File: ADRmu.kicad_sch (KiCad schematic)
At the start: 6 parts, among them J1 DIN41612_02x16_AC_EvenPins, J2 10Vf, J3 10Vs, J4 ADR, J6 return, J7 guard

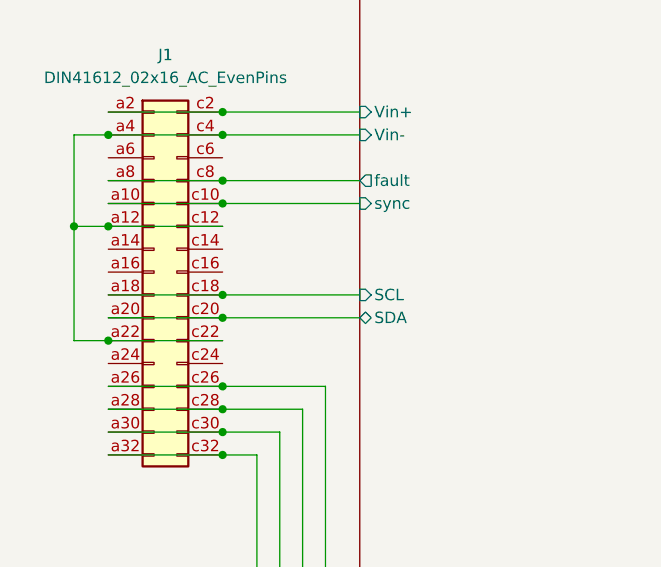
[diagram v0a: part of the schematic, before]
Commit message: asas
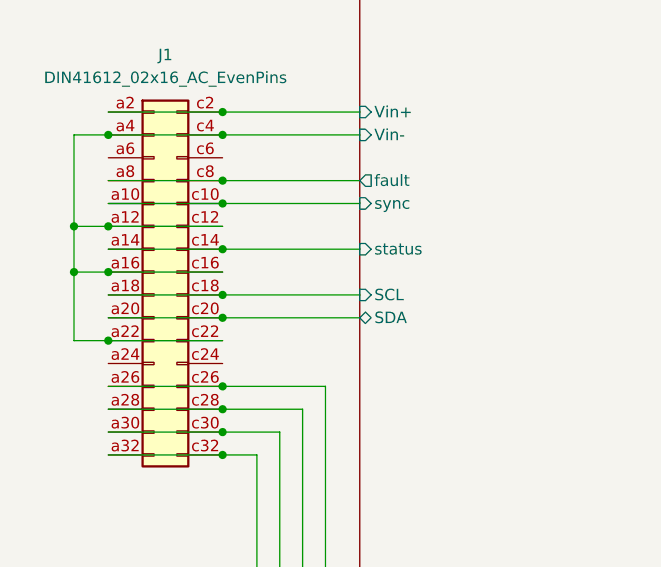
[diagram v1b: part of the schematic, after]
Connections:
- net DC-DC/Vin-: now also J1.a16 (Pin_a16), J1.c16 (Pin_c16)
- net DC-DC/status: now reaches J1.a14 (Pin_a14)
- net DC-DC/status: now also J1.c14 (Pin_c14)
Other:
- sheet DC-DC ports: added status; removed none
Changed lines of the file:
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@@
   (junction (at 68.58 82.55) (diameter 0) (color 0 0 0 0)
   )
+  (junction (at 55.88 92.71) (diameter 0) (color 0 0 0 0)
+  )
   (junction (at 55.88 100.33) (diameter 0) (color 0 0 0 0)
   )
@@
   (junction (at 68.58 105.41) (diameter 0) (color 0 0 0 0)
   )
+  (junction (at 68.58 90.17) (diameter 0) (color 0 0 0 0)
+  )
   (junction (at 68.58 85.09) (diameter 0) (color 0 0 0 0)
   )
   (junction (at 68.58 113.03) (diameter 0) (color 0 0 0 0)
   )
+  (junction (at 52.07 92.71) (diameter 0) (color 0 0 0 0)
+  )
   (junction (at 68.58 110.49) (diameter 0) (color 0 0 0 0)
   )
@@
     (stroke (width 0) (type default) (color 0 0 0 0))
   )
+  (wire (pts (xy 55.88 92.71) (xy 68.58 92.71))
+    (stroke (width 0) (type default) (color 0 0 0 0))
+  )
   (wire (pts (xy 228.6 120.65) (xy 228.6 116.84))
     (stroke (width 0) (type default) (color 0 0 0 0))
@@
     (stroke (width 0) (type default) (color 0 0 0 0))
   )
+  (wire (pts (xy 55.88 90.17) (xy 68.58 90.17))
+    (stroke (width 0) (type default) (color 0 0 0 0))
+  )
   (wire (pts (xy 55.88 77.47) (xy 52.07 77.47))
     (stroke (width 0) (type default) (color 0 0 0 0))
   )
+  (wire (pts (xy 68.58 90.17) (xy 83.82 90.17))
+    (stroke (width 0) (type default) (color 0 0 0 0))
+  )
   (wire (pts (xy 68.58 74.93) (xy 83.82 74.93))
     (stroke (width 0) (type default) (color 0 0 0 0))
@@
     (stroke (width 0) (type default) (color 0 0 0 0))
   )
+  (wire (pts (xy 52.07 92.71) (xy 52.07 100.33))
+    (stroke (width 0) (type default) (color 0 0 0 0))
+  )
   (wire (pts (xy 231.14 116.84) (xy 228.6 116.84))
     (stroke (width 0) (type default) (color 0 0 0 0))
@@
     (stroke (width 0) (type default) (color 0 0 0 0))
   )
+  (wire (pts (xy 52.07 92.71) (xy 55.88 92.71))
+    (stroke (width 0) (type default) (color 0 0 0 0))
+  )
   (wire (pts (xy 245.11 73.66) (xy 245.11 156.21))
     (stroke (width 0) (type default) (color 0 0 0 0))
@@
     (stroke (width 0) (type default) (color 0 0 0 0))
   )
-  (wire (pts (xy 52.07 87.63) (xy 52.07 100.33))
+  (wire (pts (xy 52.07 87.63) (xy 52.07 92.71))
     (stroke (width 0) (type default) (color 0 0 0 0))
   )
@@
       (effects (font (size 1.27 1.27)) (justify left))
     )
+    (pin "status" input (at 83.82 90.17 180)
+      (effects (font (size 1.27 1.27)) (justify left))
+    )
   )
   (sheet_instances
@@
     )
     (path "/b2eac6f7-6f2b-41aa-9eec-9c2e749d1013/c7e505b7-3263-497d-b6db-a745ba5df807"
-      (reference "C?") (unit 1) (value "100n") (footprint "Capacitor_SMD:C_0805_2012Metric")
+      (reference "C16") (unit 1) (value "100n") (footprint "Capacitor_SMD:C_0805_2012Metric")
+    )
+    (path "/b2eac6f7-6f2b-41aa-9eec-9c2e749d1013/f4163a13-75d2-44f7-a286-ce9ec4db0e92"
+      (reference "C17") (unit 1) (value "22u") (footprint "Capacitor_SMD:C_1206_3216Metric")
     )
     (path "/b2eac6f7-6f2b-41aa-9eec-9c2e749d1013/97a99fe4-2863-4a77-a98a-a5b1b9cc3a6a"
@@
       (reference "Q1") (unit 1) (value "Q_NPN_BCE") (footprint "Package_TO_SOT_SMD:SOT-223-3_TabPin2")
     )
+    (path "/b2eac6f7-6f2b-41aa-9eec-9c2e749d1013/1013018f-229b-406c-9517-97d026acdb9a"
+      (reference "Q2") (unit 1) (value "MMBT3904") (footprint "Package_TO_SOT_SMD:SOT-23")
+    )
     (path "/b2eac6f7-6f2b-41aa-9eec-9c2e749d1013/cf8213e3-6210-4f84-8e3b-63bd409ba25a"
       (reference "R1") (unit 1) (value "5k") (footprint "Resistor_SMD:R_0805_2012Metric")
@@
       (reference "R12") (unit 1) (value "121k") (footprint "Resistor_SMD:R_0805_2012Metric")
     )
+    (path "/027929a1-62dd-40f4-83d4-39d0de3b1543/36ed9d27-6de2-4596-b802-4666aa392e35"
+      (reference "R13") (unit 1) (value "dnp") (footprint "Resistor_SMD:R_0805_2012Metric")
+    )
+    (path "/027929a1-62dd-40f4-83d4-39d0de3b1543/e22465b8-acc1-46c4-9b5d-e2e4156397d5"
+      (reference "R14") (unit 1) (value "dnp") (footprint "Crystal:Crystal_HC52-U_Vertical")
+    )
+    (path "/027929a1-62dd-40f4-83d4-39d0de3b1543/194203bb-0c5b-44d0-b461-32ccc04431bc"
+      (reference "R15") (unit 1) (value "0") (footprint "Resistor_SMD:R_0805_2012Metric")
+    )
+    (path "/027929a1-62dd-40f4-83d4-39d0de3b1543/53cee888-d3e3-4eb2-94ea-0265cbb211bf"
+      (reference "R16") (unit 1) (value "0") (footprint "Crystal:Crystal_HC52-U_Vertical")
+    )
+    (path "/027929a1-62dd-40f4-83d4-39d0de3b1543/dfc35787-ea86-4988-ae38-87f6d9a08516"
+      (reference "R17") (unit 1) (value "0") (footprint "Resistor_SMD:R_0805_2012Metric")
+    )
+    (path "/027929a1-62dd-40f4-83d4-39d0de3b1543/15dd7c7a-30db-4890-a373-61f9b60fae6f"
+      (reference "R18") (unit 1) (value "0") (footprint "Crystal:Crystal_HC52-U_Vertical")
+    )
+    (path "/b2eac6f7-6f2b-41aa-9eec-9c2e749d1013/b6374ec4-7ed7-459e-befd-2e08e8f885b1"
+      (reference "R19") (unit 1) (value "5k") (footprint "Resistor_SMD:R_0805_2012Metric")
+    )
+    (path "/b2eac6f7-6f2b-41aa-9eec-9c2e749d1013/c704b6f6-f527-4c2e-9d83-ff759777f370"
+      (reference "R20") (unit 1) (value "200k") (footprint "Resistor_SMD:R_0805_2012Metric")
+    )
+    (path "/b2eac6f7-6f2b-41aa-9eec-9c2e749d1013/cdb664ee-3f00-4c5a-af63-9c9dadcc63d1"
+      (reference "R21") (unit 1) (value "1.8M") (footprint "Resistor_SMD:R_0805_2012Metric")
+    )
+    (path "/b2eac6f7-6f2b-41aa-9eec-9c2e749d1013/590dbea1-342c-423f-9920-ea67e378a0c1"
+      (reference "R22") (unit 1) (value "49.9k") (footprint "Resistor_SMD:R_0805_2012Metric")
+    )
     (path "/027929a1-62dd-40f4-83d4-39d0de3b1543/61e33ddb-fb2f-4483-96fd-ca725420cb1a"
